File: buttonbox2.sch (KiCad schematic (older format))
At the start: 29 parts, among them J2 AVR-PDI-6, J4 Conn_01x03_Male, SW1 SW_SP3T, SW3 Rotary_Encoder_Switch, U1 ATxmega256A3-AU, U6 AMS1117-3.3, Y2 Crystal_GND24

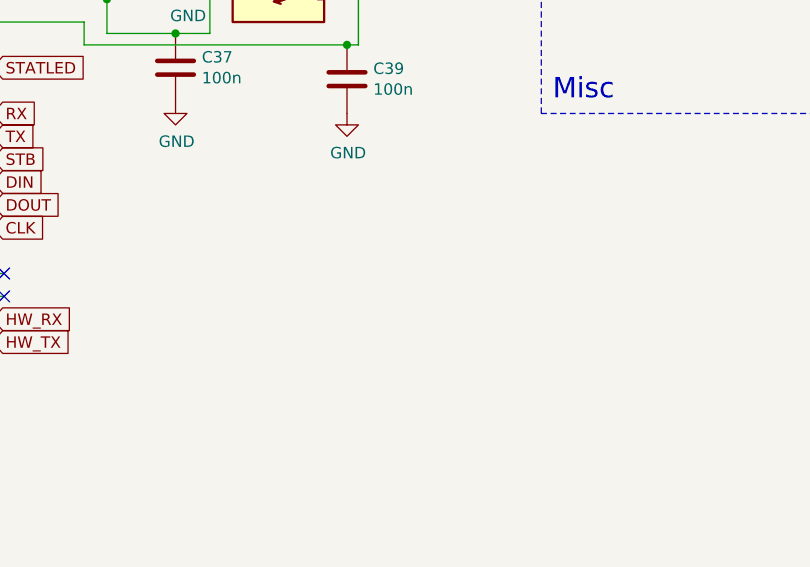
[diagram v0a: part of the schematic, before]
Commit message: Added SYS disconnect, routed USB, changed few things
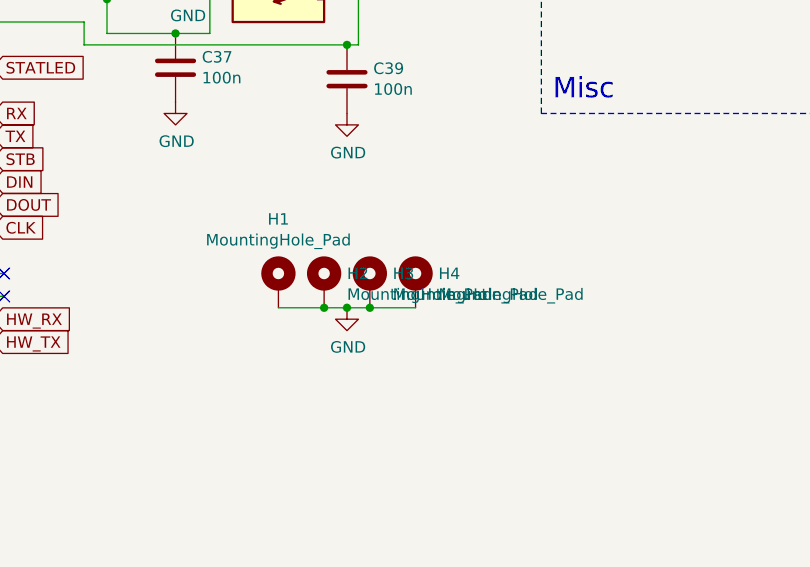
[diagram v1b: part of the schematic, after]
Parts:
- added H1, H2, H3, H4: MountingHole_Pad, MountingHole:MountingHole_2.5mm_Pad, symbol Mechanical:MountingHole_Pad
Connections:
- net GND: now also H1.1, H2.1, H3.1, H4.1
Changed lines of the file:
@@
 STB
 NoConn ~ 3300 3450
+$Comp
+L Mechanical:MountingHole_Pad H4
+U 1 1 60E727AA
+P 5150 4300
+F 0 "H4" H 5250 4349 50  0000 L CNN
+F 1 "MountingHole_Pad" H 5250 4258 50  0000 L CNN
+F 2 "MountingHole:MountingHole_2.5mm_Pad" H 5150 4300 50  0001 C CNN
+F 3 "~" H 5150 4300 50  0001 C CNN
+	1    5150 4300
+	1    0    0    -1
+$EndComp
+$Comp
+L Mechanical:MountingHole_Pad H3
+U 1 1 60E73BB2
+P 4950 4300
+F 0 "H3" H 5050 4349 50  0000 L CNN
+F 1 "MountingHole_Pad" H 5050 4258 50  0000 L CNN
+F 2 "MountingHole:MountingHole_2.5mm_Pad" H 4950 4300 50  0001 C CNN
+F 3 "~" H 4950 4300 50  0001 C CNN
+	1    4950 4300
+	1    0    0    -1
+$EndComp
+$Comp
+L Mechanical:MountingHole_Pad H2
+U 1 1 60E73E82
+P 4750 4300
+F 0 "H2" H 4850 4349 50  0000 L CNN
+F 1 "MountingHole_Pad" H 4850 4258 50  0000 L CNN
+F 2 "MountingHole:MountingHole_2.5mm_Pad" H 4750 4300 50  0001 C CNN
+F 3 "~" H 4750 4300 50  0001 C CNN
+	1    4750 4300
+	1    0    0    -1
+$EndComp
+$Comp
+L Mechanical:MountingHole_Pad H1
+U 1 1 60E7414C
+P 4550 4300
+F 0 "H1" H 4550 4587 50  0000 C CNN
+F 1 "MountingHole_Pad" H 4550 4496 50  0000 C CNN
+F 2 "MountingHole:MountingHole_2.5mm_Pad" H 4550 4300 50  0001 C CNN
+F 3 "~" H 4550 4300 50  0001 C CNN
+	1    4550 4300
+	1    0    0    -1
+$EndComp
+$Comp
+L power:GND #PWR048
+U 1 1 60E74449
+P 4850 4400
+F 0 "#PWR048" H 4850 4150 50  0001 C CNN
+F 1 "GND" H 4855 4227 50  0000 C CNN
+F 2 "" H 4850 4400 50  0001 C CNN
+F 3 "" H 4850 4400 50  0001 C CNN
+	1    4850 4400
+	1    0    0    -1
+$EndComp
+Wire Wire Line
+	4550 4400 4750 4400
+Connection ~ 4750 4400
+Wire Wire Line
+	4750 4400 4850 4400
+Connection ~ 4850 4400
+Wire Wire Line
+	4850 4400 4950 4400
+Connection ~ 4950 4400
+Wire Wire Line
+	4950 4400 5150 4400
 $EndSCHEMATC
